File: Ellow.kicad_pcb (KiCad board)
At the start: 2 copper layers, 20.5 x 38.2 mm, 26 parts, among them J1 USB_C_Receptacle_USB2.0, J2 2199119-4, J3 Conn_01x02_Female, J5 Conn_01x04_Female, Q1 A03407, Q2 A03407, U1 AP2112K-3.3, U2 E73-2G4M08S1C, U3 LN2054Y42AMR, Y1 32.768kHz

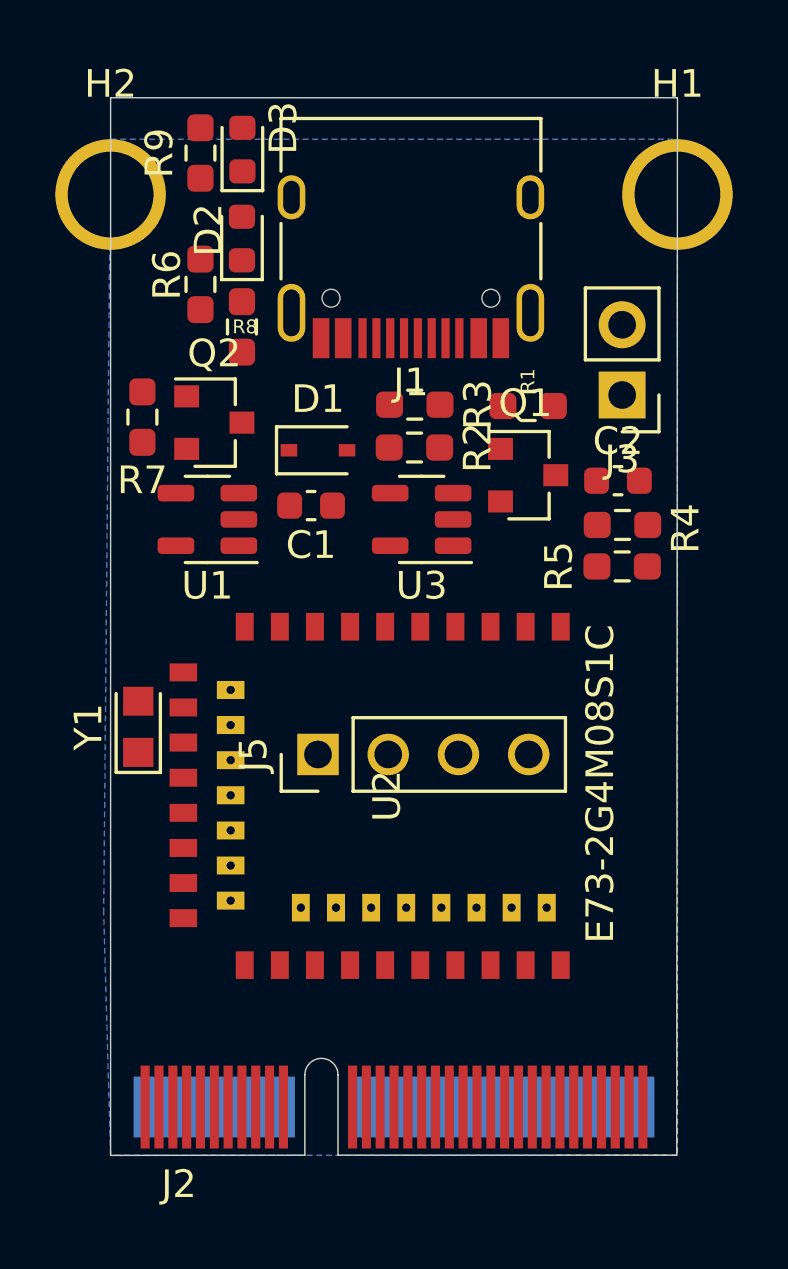
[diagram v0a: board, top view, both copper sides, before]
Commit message: routed and ready for QA check
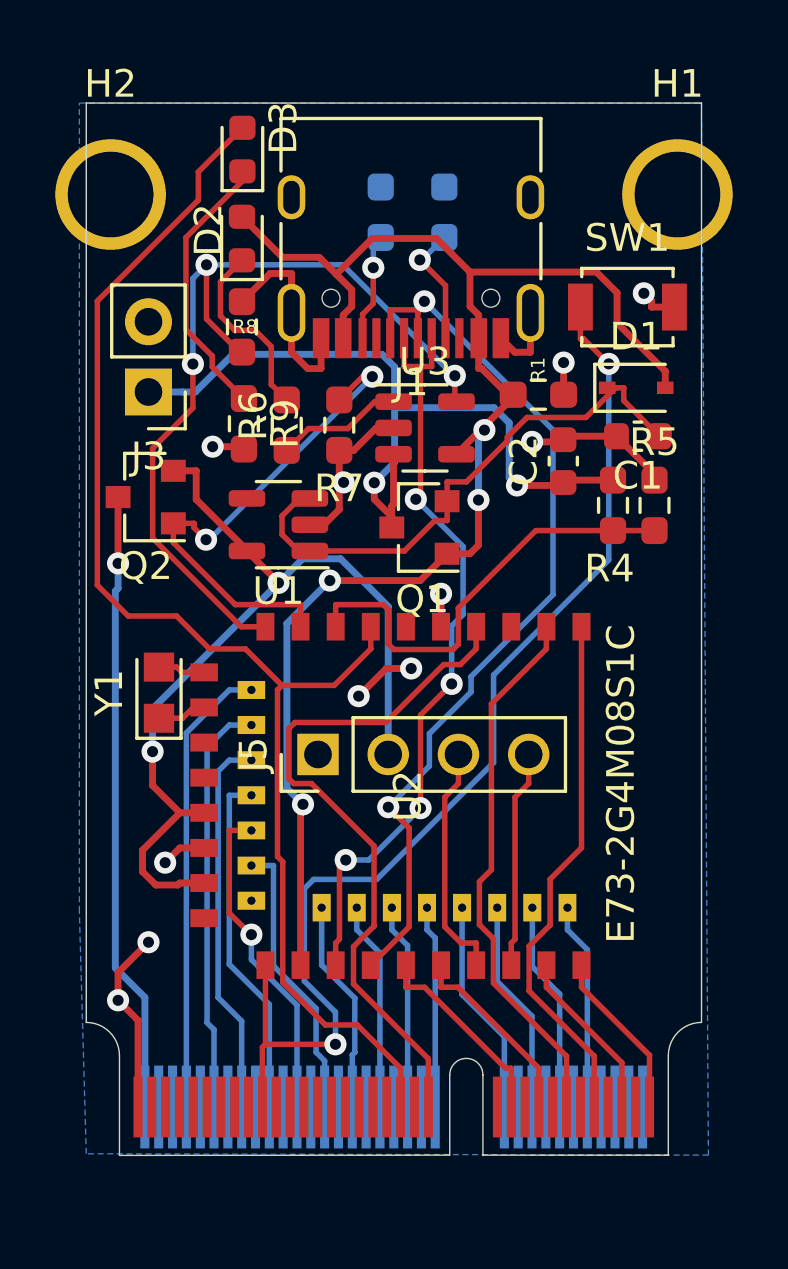
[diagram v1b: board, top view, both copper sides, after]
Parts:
- added SW1: SW_Push, Button_Switch_SMD:SW_SPST_B3U-1000P, F.Cu at (244.0, 100.1)
- J2, R2, R3: moved to B.Cu
- moved J3 17.1 mm to (226.7, 103.2)
- moved C1 12.1 mm to (244.4, 104.8)
- moved D1 11.7 mm to (244.3, 103.1)
- moved R9 9.92 mm to (230.1, 104.4), turned to 270 degrees
- moved R2 8.58 mm to (237.4, 96.7), turned to 90 degrees
- moved R7 7.13 mm to (233.6, 104.4)
- moved R3 7.07 mm to (235.1, 96.7), turned to 90 degrees
- moved R6 5.97 mm to (231.7, 104.4)
- moved Q1 4.36 mm to (236.5, 108.1), turned to 180 degrees
- moved Q2 3.66 mm to (226.6, 107.0), turned to 180 degrees
- moved U3 3.31 mm to (236.7, 104.5), turned to 0 degrees
- moved U1 2.58 mm to (231.4, 108.0)
- moved R5 2.50 mm to (245.0, 107.3), turned to 90 degrees
- moved C2 2.10 mm to (241.7, 105.7), turned to 90 degrees
- moved Y1 1.44 mm to (227.0, 114.1)
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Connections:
- J1 pad A8: Net-(J1-PadA8) -> (no net)
- J1 pad B8: Net-(J1-PadB8) -> (no net)
- J2 pad 1: Net-(J2-Pad1) -> P0.10
- J2 pad 10: Net-(J2-Pad10) -> P1.06
- J2 pad 11: Net-(J2-Pad11) -> (no net)
- J2 pad 12: Net-(J2-Pad12) -> (no net)
- J2 pad 13: Net-(J2-Pad13) -> P1.10
- J2 pad 14: Net-(J2-Pad14) -> P1.04
- J2 pad 15: P0.26 -> (no net)
- J2 pad 16: Net-(J2-Pad16) -> (no net)
- J2 pad 17: Net-(J2-Pad17) -> P0.24
- J2 pad 18: Net-(J2-Pad18) -> P1.02
- J2 pad 19: P0.06 -> (no net)
- J2 pad 2: EXT_VCC -> (no net)
- J2 pad 20: Net-(J2-Pad20) -> (no net)
- J2 pad 21: Net-(J2-Pad21) -> P0.13
- J2 pad 22: Net-(J2-Pad22) -> P1.00
- J2 pad 23: P0.08 -> (no net)
- J2 pad 3: Net-(J2-Pad3) -> (no net)
- J2 pad 32: Net-(J2-Pad32) -> P0.22
- J2 pad 33: Net-(J2-Pad33) -> P0.28
- J2 pad 34: Net-(J2-Pad34) -> (no net)
- J2 pad 35: P0.04 -> (no net)
- J2 pad 36: Net-(J2-Pad36) -> P0.20
- J2 pad 37: Net-(J2-Pad37) -> P0.02
- J2 pad 38: P0.02 -> (no net)
- J2 pad 39: P0.12 -> (no net)
- J2 pad 4: Net-(J2-Pad4) -> (no net)
- J2 pad 40: Net-(J2-Pad40) -> P0.17
- J2 pad 41: Net-(J2-Pad41) -> (no net)
- J2 pad 42: RESET -> (no net)
- J2 pad 43: P0.07 -> (no net)
- J2 pad 44: Net-(J2-Pad44) -> P0.15
- J2 pad 45: Net-(J2-Pad45) -> (no net)
- J2 pad 46: P0.28 -> (no net)
- J2 pad 47: P0.15 -> (no net)
- J2 pad 48: Net-(J2-Pad48) -> P0.07
- J2 pad 49: Net-(J2-Pad49) -> (no net)
- J2 pad 5: Net-(J2-Pad5) -> P0.09
- J2 pad 50: P0.03 -> (no net)
- J2 pad 51: P0.17 -> (no net)
- J2 pad 52: Net-(J2-Pad52) -> P0.12
- J2 pad 53: Net-(J2-Pad53) -> (no net)
- J2 pad 54: P0.13 -> (no net)
- J2 pad 55: P0.20 -> (no net)
- J2 pad 56: Net-(J2-Pad56) -> P0.04
- J2 pad 57: Net-(J2-Pad57) -> RESET
- J2 pad 58: P0.24 -> (no net)
- J2 pad 59: P0.22 -> (no net)
- J2 pad 6: GND -> (no net)
- J2 pad 60: Net-(J2-Pad60) -> P0.08
- J2 pad 61: Net-(J2-Pad61) -> (no net)
- J2 pad 62: P1.10 -> (no net)
- J2 pad 63: P1.00 -> (no net)
- J2 pad 64: Net-(J2-Pad64) -> P0.06
- J2 pad 65: Net-(J2-Pad65) -> (no net)
- J2 pad 66: P1.11 -> (no net)
- J2 pad 67: P1.02 -> (no net)
- J2 pad 68: Net-(J2-Pad68) -> P0.26
- J2 pad 69: Net-(J2-Pad69) -> (no net)
- J2 pad 7: Net-(J2-Pad7) -> (no net)
- J2 pad 70: P0.09 -> (no net)
- J2 pad 71: P1.04 -> (no net)
- J2 pad 72: Net-(J2-Pad72) -> (no net)
- J2 pad 73: Net-(J2-Pad73) -> (no net)
- J2 pad 74: P0.10 -> EXT_VCC
- J2 pad 75: P1.06 -> GND
- J2 pad 8: Net-(J2-Pad8) -> (no net)
- J2 pad 9: Net-(J2-Pad9) -> P1.11
- U1 pad 4: Net-(U1-Pad4) -> (no net)
- U2 pad 15: P0.05 -> (no net)
- U2 pad 17: P1.09 -> (no net)
- U2 pad 25: DCCH -> (no net)
- U2 pad 3: P0.03 -> (no net)
- U2 pad 6: P1.13 -> (no net)
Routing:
- net VBUS: track 0.00 -> 55.9 mm, vias 0 -> 4
- net P0.02: track 0.00 -> 49.3 mm
- net RESET: track 0.00 -> 41.2 mm, vias 0 -> 2
- net GND: track 0.00 -> 37.0 mm, vias 0 -> 11
- net VDD_H: track 0.00 -> 33.1 mm, vias 0 -> 2
- net DATA+: track 0.00 -> 32.7 mm, vias 0 -> 2
- net PROG: track 0.00 -> 31.4 mm, vias 0 -> 3
- net VBAT: track 0.00 -> 28.6 mm, vias 0 -> 2
- net DATA-: track 0.00 -> 27.9 mm, vias 0 -> 4
- net P0.28: track 0.00 -> 25.5 mm
- net EXT_VCC: track 0.00 -> 22.5 mm, vias 0 -> 1
- net Net-(C1-Pad1): track 0.00 -> 20.5 mm
- net P1.10: track 0.00 -> 19.7 mm
- net P1.11: track 0.00 -> 19.1 mm
- net EXT_VCC_CONTROL: track 0.00 -> 18.5 mm, vias 0 -> 2
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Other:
- board size 20.5 x 38.2 mm -> 22.2 x 38.1 mm
- net class Power added: clearance 0.25, trace_width 0.25, via_dia 0.8, via_drill 0.4
